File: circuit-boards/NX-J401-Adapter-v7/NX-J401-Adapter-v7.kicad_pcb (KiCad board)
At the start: 4 copper layers, 120.3 x 79 mm, 135 parts, among them J1 Terminal, J10 POWER, J11 USB_C_Receptacle_USB2.0_14P, J2 Terminal, J3 NX CONTROL & UART, J4 15V, J5 NX CONTROL & UART, J6 NX CONTROL & UART, J7 USB1, J8 SWD, J9 CAN1, Q1 CSD19534Q5A, Q2 SI2301CDS-T1-GE3, Q3 CSD17578Q5A, Q4 CSD17578Q5A, Q5 SS8050, Q6 CSD19534Q5A, Q7 SI2301CDS-T1-GE3, Q8 CSD19534Q5A, Q9 CSD19534Q5A, SW1 RESET, SW2 RECOVERY, U1 LM74700QDBVRQ1, U2 TPS613222ADBV, U3 STM32G431CBTx, U5 ISO6721BDR, U6 FT232RNL, U7 LM74700QDBVRQ1, U8 TJA1051T/3/1J

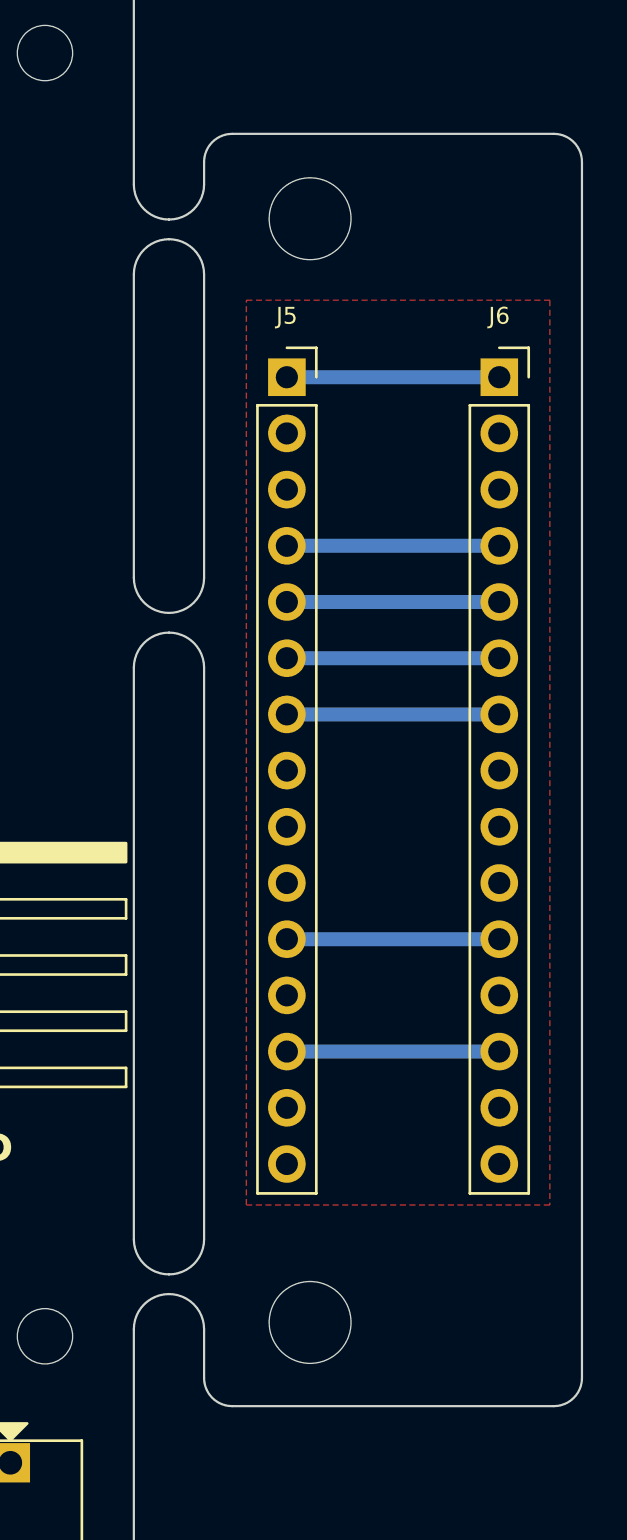
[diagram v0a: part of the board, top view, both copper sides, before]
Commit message: PCB update
Signed-off-by: Scott Berman <sgberman1@gmail.com>
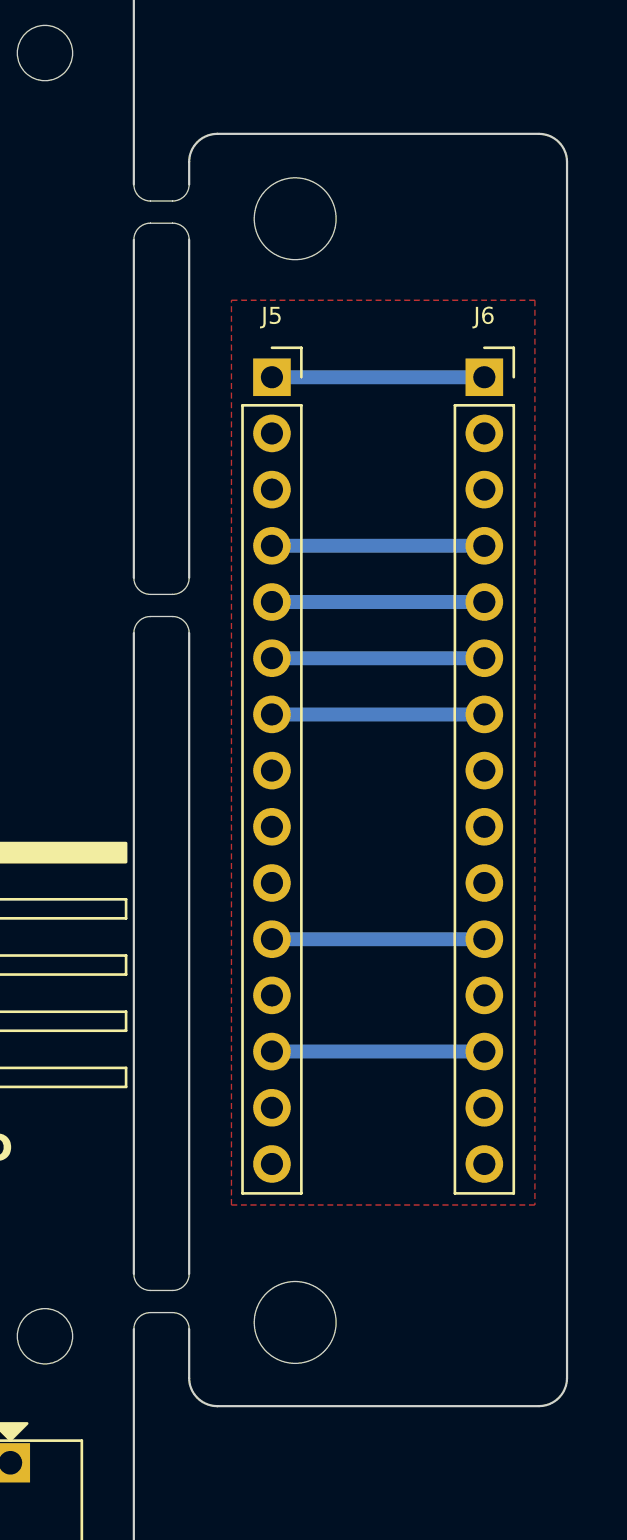
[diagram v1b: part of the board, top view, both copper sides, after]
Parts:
- LP1, LP2, LP3, LP4: value ~ -> Light Pipe
- U4: value ~ -> LM5176PWPR
- moved H3 0.68 mm to (263.3, 86.0)
- moved H4 0.68 mm to (263.3, 135.9)
- moved J5 0.68 mm to (262.2, 93.1)
- moved J6 0.68 mm to (271.8, 93.1)
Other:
- board size 120.3 x 79 mm -> 119.6 x 79 mm
